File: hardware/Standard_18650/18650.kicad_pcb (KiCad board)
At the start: 2 copper layers, 104.3 x 16 mm, 58 parts, among them J2 Battery, J3 GPIO, J4 USB_B_Micro, J5 Power, J6 LEDs, J7 GPIO, Q1 BSS806N, Q2 BSS806N, Q3 BSS806N, Q4 BSS806N, SW1 Mode, SW2 Power, U1 STM32F411CE, U2 AP2210N-3.3TRG1, U3 MCP73830, U4 ESD7002WTT1G, U5 GD25Q16CEIGR, Y1 24Mhz

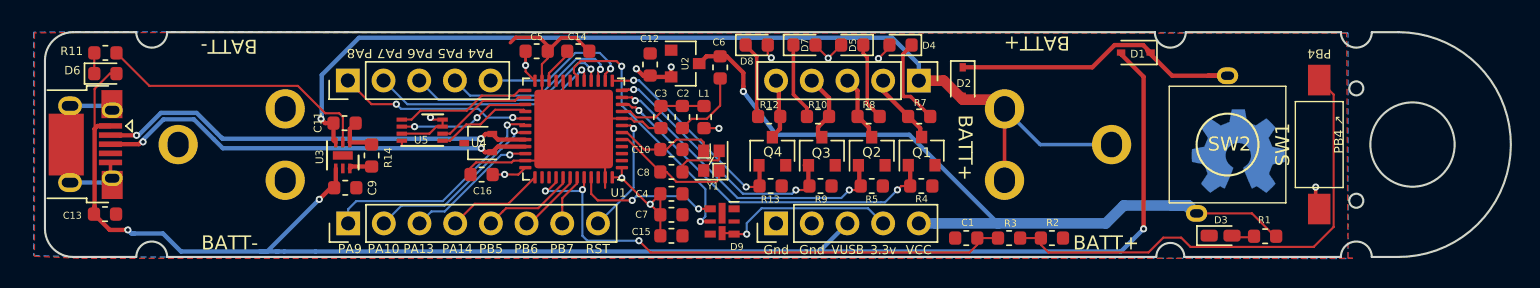
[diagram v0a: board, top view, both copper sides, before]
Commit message: Checkpoint commit (v1.2a3)
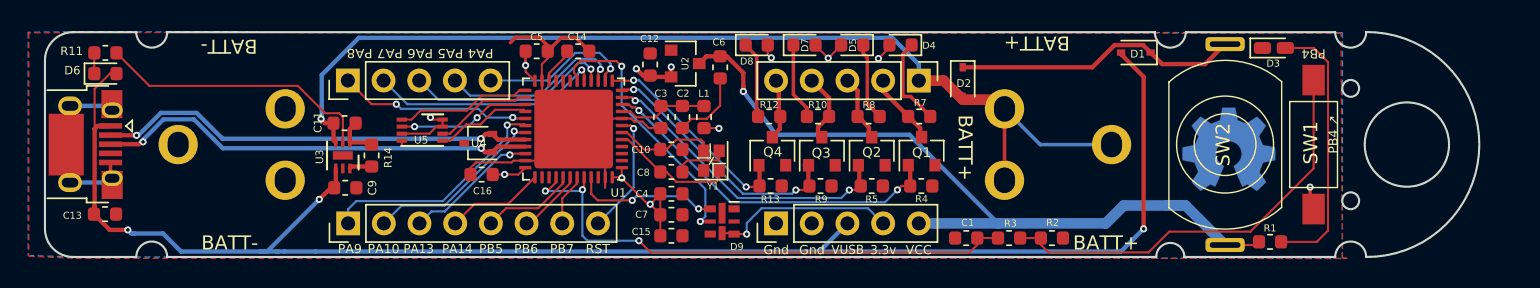
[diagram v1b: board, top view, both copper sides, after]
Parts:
- SW2: footprint Jeremy:Switch_L068-A-DC30V1A -> Jeremy Button/Switch:SW_KAN-15_PHT
- moved D3 13.9 mm to (145.6, 93.1)
- moved REF** 0.69 mm to (142.4, 100.3)
- moved R1 0.53 mm to (145.3, 106.9), turned to 180 degrees
- moved SW1 0.40 mm to (148.4, 100.0)
- moved SW2 0.18 mm to (142.1, 100.0), turned to 270 degrees
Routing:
- net Net-(D3-Pad2): track 1.59 -> 19.1 mm
- net Net-(R2-Pad1): track 35.2 -> 30.4 mm
- net /VIN: track 57.5 -> 54.5 mm
- net Net-(D1-Pad1): track 22.0 -> 20.5 mm
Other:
- board size 104.3 x 16 mm -> 102.1 x 16 mm
- board text added: "v1.2a3"
- board text removed: "v1.2a2"
